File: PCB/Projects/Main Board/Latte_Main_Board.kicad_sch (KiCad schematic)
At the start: 119 parts, among them J1 SM02B-SURS-TF_LF__SN_, J2 SM02B-SURS-TF_LF__SN_, J3 Molex 505110-0892, J4 Molex 505110-0592, J5 Molex 505110-0892, J6 Molex 505110-0592, J8 Conn_01x04_Pin, J9 Molex 505110-1792, Q1 MMBT2222A, Q2 MMBT2222A, SW1 SW_Push, SW2 SW_Push, SW3 SW_Push, SW4 SW_Push, SW5 SW_Push, SW6 SW_Push, SW7 SW_Push, SW8 SW_Push, U1 HAL4395, U10 HAL4395, U11 HAL4395, U2 RP2350_80QFN, U3 HAL4395, U4 ST_LSM6, U5 ST_LSM6, U6 HAL4395, U7 HAL4395, U8 HAL4395, U9 HAL4395, Y1 ABM8-272-T3

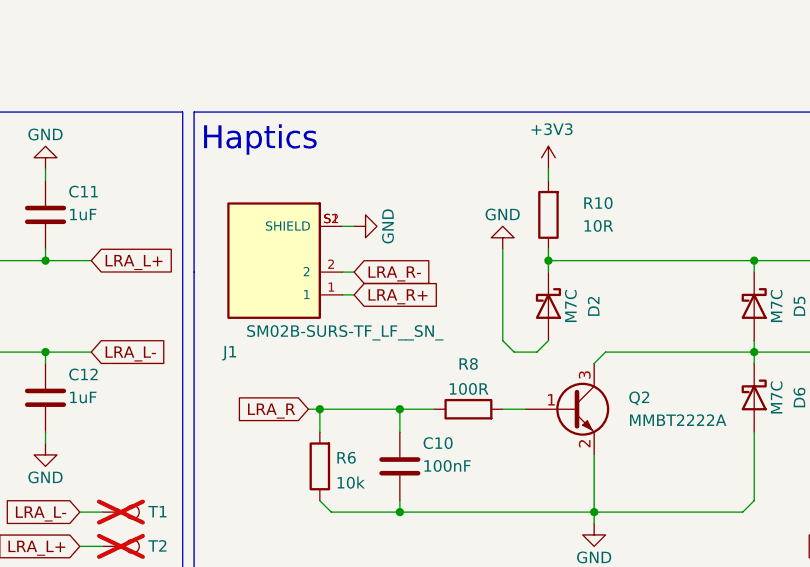
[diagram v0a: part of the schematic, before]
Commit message: Routing Updates
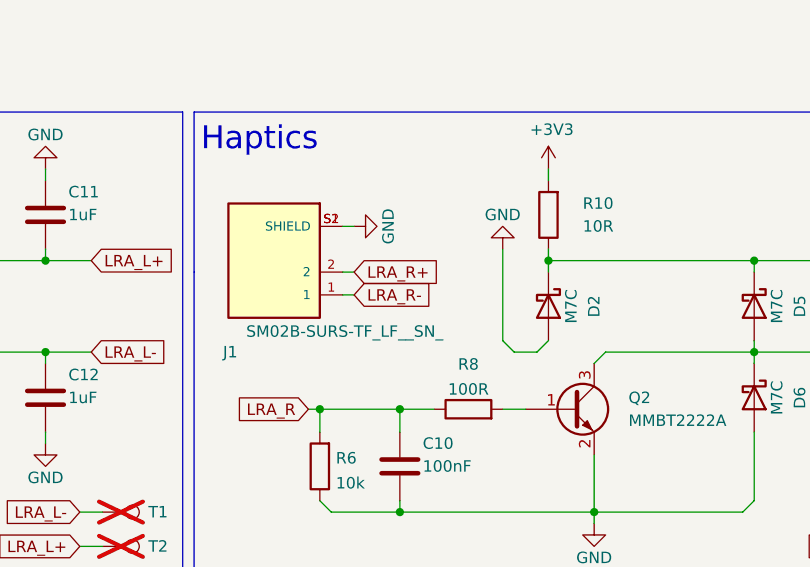
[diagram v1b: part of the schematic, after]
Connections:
- net LRA_R+: now also J1.2; no longer J1.1
- net LRA_R-: now also J1.1; no longer J1.2
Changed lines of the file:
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@@
 	(global_label "LRA_R-"
 		(shape input)
+		(at 302.26 34.29 0)
+		(fields_autoplaced yes)
+		(effects
+			(font
+				(size 1.27 1.27)
+			)
+			(justify left)
+		)
+		(property "Intersheetrefs" "${INTERSHEET_REFS}"
+			(at 312.4419 34.29 0)
+			(effects
+				(font
+					(size 1.27 1.27)
+				)
+				(justify left)
+				(hide yes)
+			)
+		)
+	)
+	(global_label "ADC_2"
+		(shape input)
+		(at 139.7 -36.83 0)
+		(fields_autoplaced yes)
+		(effects
+			(font
+				(size 1.27 1.27)
+			)
+			(justify left)
+		)
+		(property "Intersheetrefs" "${INTERSHEET_REFS}"
+			(at 148.4909 -36.83 0)
+			(effects
+				(font
+					(size 1.27 1.27)
+				)
+				(justify left)
+				(hide yes)
+			)
+		)
+	)
+	(global_label "I2C1_SCL"
+		(shape input)
+		(at 204.47 130.81 0)
+		(fields_autoplaced yes)
+		(effects
+			(font
+				(size 1.27 1.27)
+			)
+			(justify left)
+		)
+		(property "Intersheetrefs" "${INTERSHEET_REFS}"
+			(at 216.2242 130.81 0)
+			(effects
+				(font
+					(size 1.27 1.27)
+				)
+				(justify left)
+				(hide yes)
+			)
+		)
+	)
+	(global_label "WL_CLK"
+		(shape input)
+		(at 148.59 139.7 0)
+		(fields_autoplaced yes)
+		(effects
+			(font
+				(size 1.27 1.27)
+			)
+			(justify left)
+		)
+		(property "Intersheetrefs" "${INTERSHEET_REFS}"
+			(at 157.9362 139.7 0)
+			(effects
+				(font
+					(size 1.27 1.27)
+				)
+				(justify left)
+				(hide yes)
+			)
+		)
+	)
+	(global_label "SPI1_RX"
+		(shape input)
+		(at 441.96 113.03 180)
+		(fields_autoplaced yes)
+		(effects
+			(font
+				(size 1.27 1.27)
+			)
+			(justify right)
+		)
+		(property "Intersheetrefs" "${INTERSHEET_REFS}"
+			(at 431.2339 113.03 0)
+			(effects
+				(font
+					(size 1.27 1.27)
+				)
+				(justify right)
+				(hide yes)
+			)
+		)
+	)
+	(global_label "STICK_R_RGB_OUT"
+		(shape input)
+		(at 290.83 227.33 180)
+		(fields_autoplaced yes)
+		(effects
+			(font
+				(size 1.27 1.27)
+			)
+			(justify right)
+		)
+		(property "Intersheetrefs" "${INTERSHEET_REFS}"
+			(at 270.9115 227.33 0)
+			(effects
+				(font
+					(size 1.27 1.27)
+				)
+				(justify right)
+				(hide yes)
+			)
+		)
+	)
+	(global_label "N_DATA_3.3"
+		(shape input)
+		(at 204.47 128.27 0)
+		(fields_autoplaced yes)
+		(effects
+			(font
+				(size 1.27 1.27)
+			)
+			(justify left)
+		)
+		(property "Intersheetrefs" "${INTERSHEET_REFS}"
+			(at 217.4985 128.3494 0)
+			(effects
+				(font
+					(size 1.27 1.27)
+				)
+				(justify left)
+				(hide yes)
+			)
+		)
+	)
+	(global_label "SWD"
+		(shape input)
+		(at 73.66 189.23 180)
+		(fields_autoplaced yes)
+		(effects
+			(font
+				(size 1.27 1.27)
+			)
+			(justify right)
+		)
+		(property "Intersheetrefs" "${INTERSHEET_REFS}"
+			(at 66.7439 189.23 0)
+			(effects
+				(font
+					(size 1.27 1.27)
+				)
+				(justify right)
+				(hide yes)
+			)
+		)
+	)
+	(global_label "I2C1_SDA"
+		(shape input)
+		(at 443.23 90.17 270)
+		(fields_autoplaced yes)
+		(effects
+			(font
+				(size 1.27 1.27)
+			)
+			(justify right)
+		)
+		(property "Intersheetrefs" "${INTERSHEET_REFS}"
+			(at 443.23 101.3305 90)
+			(effects
+				(font
+					(size 1.27 1.27)
+				)
+				(justify right)
+				(hide yes)
+			)
+		)
+	)
+	(global_label "ADC_0"
+		(shape input)
+		(at 139.7 -72.39 0)
+		(fields_autoplaced yes)
+		(effects
+			(font
+				(size 1.27 1.27)
+			)
+			(justify left)
+		)
+		(property "Intersheetrefs" "${INTERSHEET_REFS}"
+			(at 148.4909 -72.39 0)
+			(effects
+				(font
+					(size 1.27 1.27)
+				)
+				(justify left)
+				(hide yes)
+			)
+		)
+	)
+	(global_label "LRA_L"
+		(shape input)
+		(at 157.48 152.4 0)
+		(fields_autoplaced yes)
+		(effects
+			(font
+				(size 1.27 1.27)
+			)
+			(justify left)
+		)
+		(property "Intersheetrefs" "${INTERSHEET_REFS}"
+			(at 165.8476 152.4 0)
+			(effects
+				(font
+					(size 1.27 1.27)
+				)
+				(justify left)
+				(hide yes)
+			)
+		)
+	)
+	(global_label "LRA_R+"
+		(shape input)
 		(at 302.26 31.75 0)
 		(fields_autoplaced yes)
@@
 			(effects
 				(font
-					(size 1.27 1.27)
-				)
-				(justify left)
-				(hide yes)
-			)
-		)
-	)
-	(global_label "ADC_2"
-		(shape input)
-		(at 139.7 -36.83 0)
-		(fields_autoplaced yes)
-		(effects
-			(font
-				(size 1.27 1.27)
-			)
-			(justify left)
-		)
-		(property "Intersheetrefs" "${INTERSHEET_REFS}"
-			(at 148.4909 -36.83 0)
-			(effects
-				(font
-					(size 1.27 1.27)
-				)
-				(justify left)
-				(hide yes)
-			)
-		)
-	)
-	(global_label "I2C1_SCL"
-		(shape input)
-		(at 204.47 130.81 0)
-		(fields_autoplaced yes)
-		(effects
-			(font
-				(size 1.27 1.27)
-			)
-			(justify left)
-		)
-		(property "Intersheetrefs" "${INTERSHEET_REFS}"
-			(at 216.2242 130.81 0)
-			(effects
-				(font
-					(size 1.27 1.27)
-				)
-				(justify left)
-				(hide yes)
-			)
-		)
-	)
-	(global_label "WL_CLK"
-		(shape input)
-		(at 148.59 139.7 0)
-		(fields_autoplaced yes)
-		(effects
-			(font
-				(size 1.27 1.27)
-			)
-			(justify left)
-		)
-		(property "Intersheetrefs" "${INTERSHEET_REFS}"
-			(at 157.9362 139.7 0)
-			(effects
-				(font
-					(size 1.27 1.27)
-				)
-				(justify left)
-				(hide yes)
-			)
-		)
-	)
-	(global_label "SPI1_RX"
-		(shape input)
-		(at 441.96 113.03 180)
-		(fields_autoplaced yes)
-		(effects
-			(font
-				(size 1.27 1.27)
-			)
-			(justify right)
-		)
-		(property "Intersheetrefs" "${INTERSHEET_REFS}"
-			(at 431.2339 113.03 0)
-			(effects
-				(font
-					(size 1.27 1.27)
-				)
-				(justify right)
-				(hide yes)
-			)
-		)
-	)
-	(global_label "STICK_R_RGB_OUT"
-		(shape input)
-		(at 290.83 227.33 180)
-		(fields_autoplaced yes)
-		(effects
-			(font
-				(size 1.27 1.27)
-			)
-			(justify right)
-		)
-		(property "Intersheetrefs" "${INTERSHEET_REFS}"
-			(at 270.9115 227.33 0)
-			(effects
-				(font
-					(size 1.27 1.27)
-				)
-				(justify right)
-				(hide yes)
-			)
-		)
-	)
-	(global_label "N_DATA_3.3"
-		(shape input)
-		(at 204.47 128.27 0)
-		(fields_autoplaced yes)
-		(effects
-			(font
-				(size 1.27 1.27)
-			)
-			(justify left)
-		)
-		(property "Intersheetrefs" "${INTERSHEET_REFS}"
-			(at 217.4985 128.3494 0)
-			(effects
-				(font
-					(size 1.27 1.27)
-				)
-				(justify left)
-				(hide yes)
-			)
-		)
-	)
-	(global_label "SWD"
-		(shape input)
-		(at 73.66 189.23 180)
-		(fields_autoplaced yes)
-		(effects
-			(font
-				(size 1.27 1.27)
-			)
-			(justify right)
-		)
-		(property "Intersheetrefs" "${INTERSHEET_REFS}"
-			(at 66.7439 189.23 0)
-			(effects
-				(font
-					(size 1.27 1.27)
-				)
-				(justify right)
-				(hide yes)
-			)
-		)
-	)
-	(global_label "I2C1_SDA"
-		(shape input)
-		(at 443.23 90.17 270)
-		(fields_autoplaced yes)
-		(effects
-			(font
-				(size 1.27 1.27)
-			)
-			(justify right)
-		)
-		(property "Intersheetrefs" "${INTERSHEET_REFS}"
-			(at 443.23 101.3305 90)
-			(effects
-				(font
-					(size 1.27 1.27)
-				)
-				(justify right)
-				(hide yes)
-			)
-		)
-	)
-	(global_label "ADC_0"
-		(shape input)
-		(at 139.7 -72.39 0)
-		(fields_autoplaced yes)
-		(effects
-			(font
-				(size 1.27 1.27)
-			)
-			(justify left)
-		)
-		(property "Intersheetrefs" "${INTERSHEET_REFS}"
-			(at 148.4909 -72.39 0)
-			(effects
-				(font
-					(size 1.27 1.27)
-				)
-				(justify left)
-				(hide yes)
-			)
-		)
-	)
-	(global_label "LRA_L"
-		(shape input)
-		(at 157.48 152.4 0)
-		(fields_autoplaced yes)
-		(effects
-			(font
-				(size 1.27 1.27)
-			)
-			(justify left)
-		)
-		(property "Intersheetrefs" "${INTERSHEET_REFS}"
-			(at 165.8476 152.4 0)
-			(effects
-				(font
-					(size 1.27 1.27)
-				)
-				(justify left)
-				(hide yes)
-			)
-		)
-	)
-	(global_label "LRA_R+"
-		(shape input)
-		(at 302.26 34.29 0)
-		(fields_autoplaced yes)
-		(effects
-			(font
-				(size 1.27 1.27)
-			)
-			(justify left)
-		)
-		(property "Intersheetrefs" "${INTERSHEET_REFS}"
-			(at 312.4419 34.29 0)
-			(effects
-				(font

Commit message: Routing updates
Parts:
- U4, U5: LCSC C784817 -> C126672; MPN LSM6DSRTR -> LSM6DSLTR
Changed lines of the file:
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@@
 			)
 		)
-		(property "LCSC" "C784817"
+		(property "LCSC" "C126672"
 			(at 453.39 156.21 0)
 			(effects
@@
 			)
 		)
-		(property "MPN" "LSM6DSRTR"
+		(property "MPN" "LSM6DSLTR"
 			(at 453.39 156.21 0)
 			(effects
@@
 			)
 		)
-		(property "LCSC" "C784817"
+		(property "LCSC" "C126672"
 			(at 453.39 116.84 0)
 			(effects
@@
 			)
 		)
-		(property "MPN" "LSM6DSRTR"
+		(property "MPN" "LSM6DSLTR"
 			(at 453.39 116.84 0)
 			(effects
